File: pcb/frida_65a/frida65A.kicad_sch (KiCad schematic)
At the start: 44 parts, among them J1 CONN_PWR, J10 TP_LOGIC, J11 TP_OUT, J2 CONN_IN_P, J3 CONN_IN_N, J4 TP_CFG, J5 CONN_CFG, J6 TP_IN, J7 TP_INIT, J8 TP_SAMP, J9 TP_COMP, U1 DUT

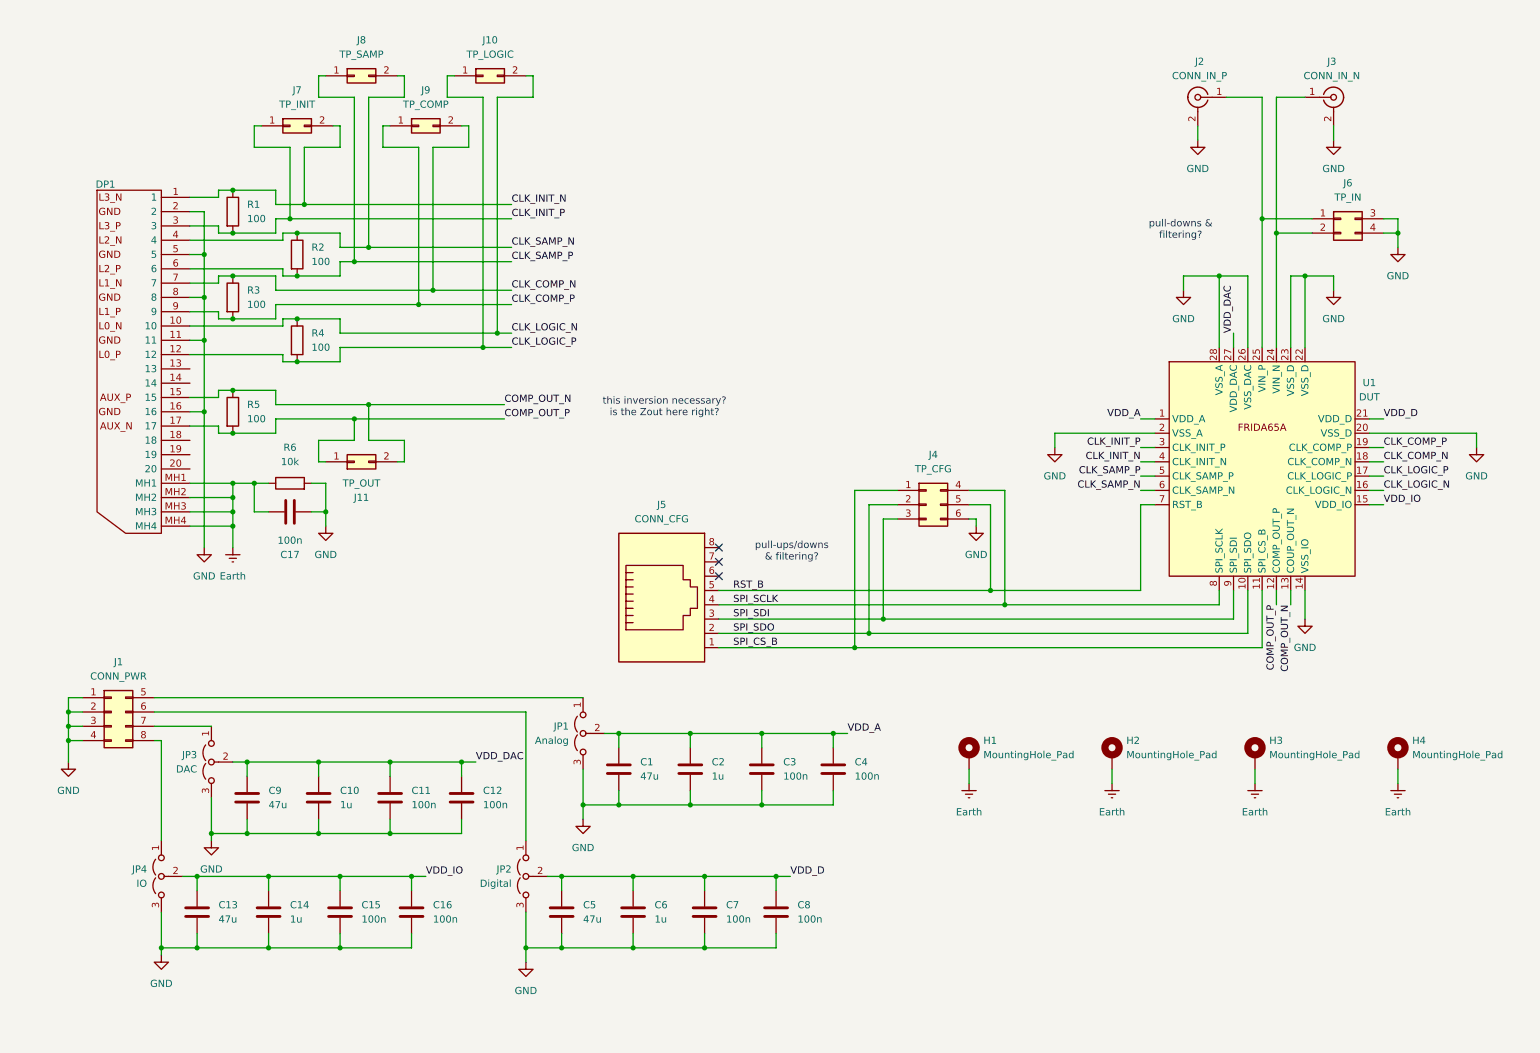
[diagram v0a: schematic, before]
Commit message: Update pcb
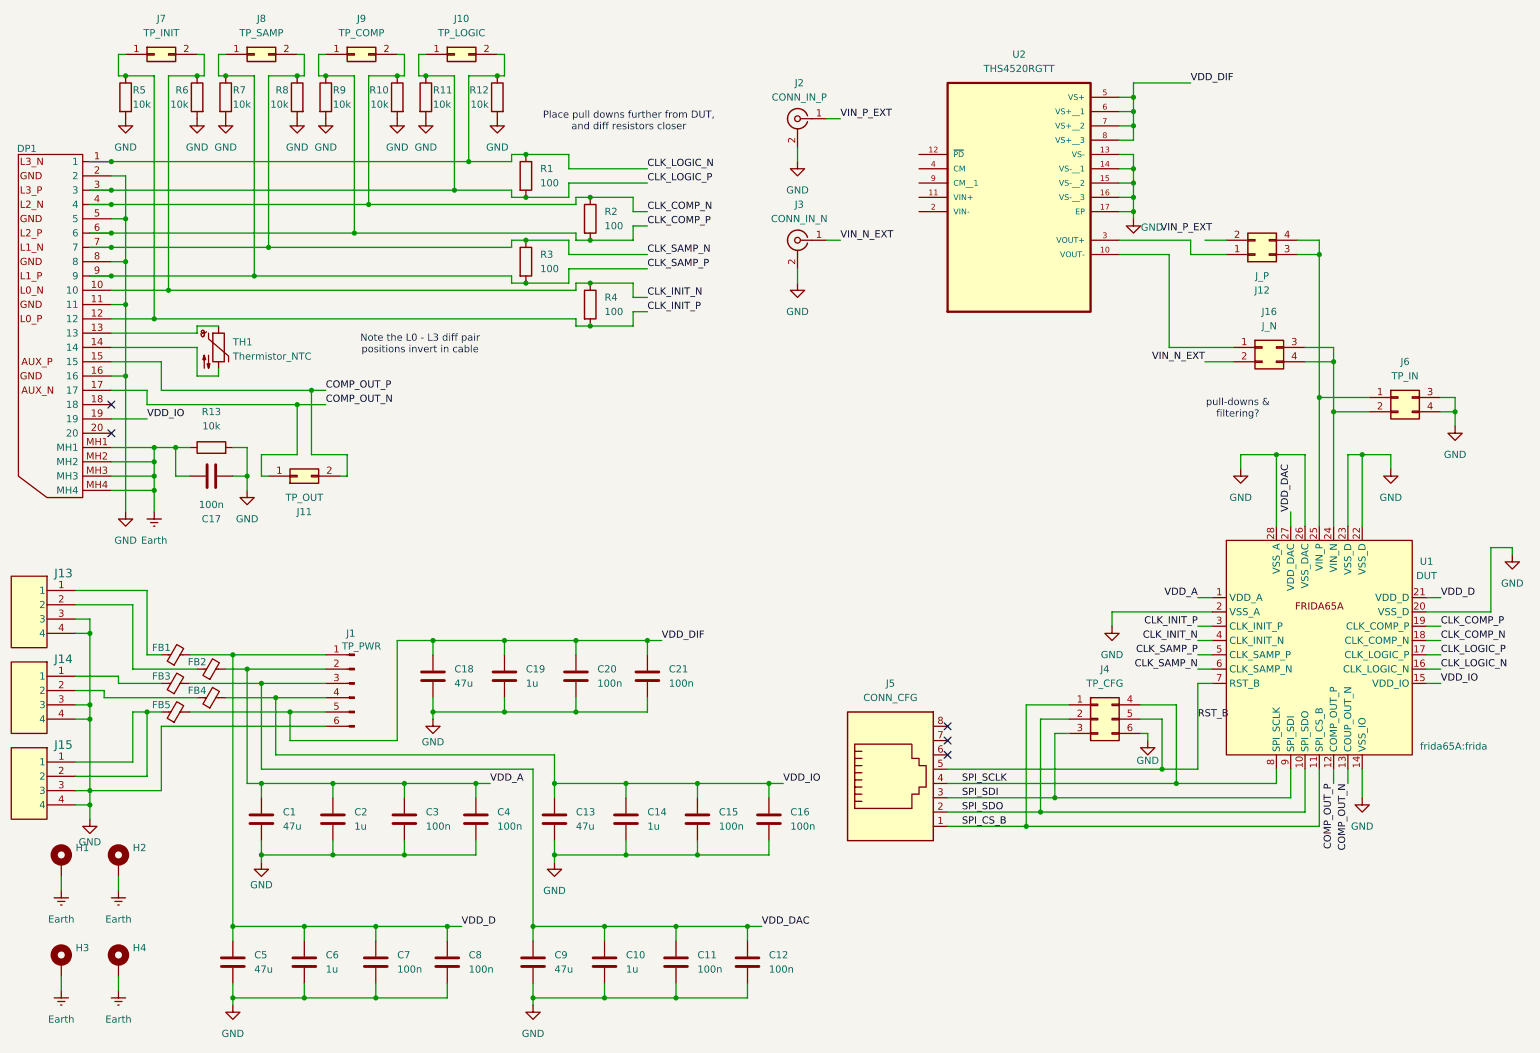
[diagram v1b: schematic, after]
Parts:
- removed J1: CONN_PWR, Silab:Molex_Mini-Fit_Jr_02x04_horizontal, symbol silab:Molex_02x04_Mini-Fit_Jr
- removed JP1: Analog, symbol Jumper:Jumper_3_Open
- removed JP2: Digital, symbol Jumper:Jumper_3_Open
- removed JP3: DAC, symbol Jumper:Jumper_3_Open
- removed JP4: IO, symbol Jumper:Jumper_3_Open
- added C18: 47u, Capacitor_SMD:C_0603_1608Metric, symbol Device:C
- added C19: 1u, Capacitor_SMD:C_0603_1608Metric, symbol Device:C
- added C20, C21: 100n, Capacitor_SMD:C_0603_1608Metric, symbol Device:C
- added FB1, FB2, FB3, FB4, FB5: FerriteBead_Small, Resistor_SMD:R_0603_1608Metric, symbol Device:FerriteBead_Small
- added J1: TP_PWR, Silab:Molex_Mini-Fit_Jr_02x04_horizontal, symbol Connector:Conn_01x06_Pin
- added J12: J_P, symbol Connector_Generic:Conn_02x02_Top_Bottom
- added J13, J14, J15: 469914004, CONN_SD-46991-001_04_MOL, symbol frida:469914004
- added J16: J_N, symbol Connector_Generic:Conn_02x02_Top_Bottom
- added R10, R11, R12, R6, R7, R8, R9: 10k, Resistor_SMD:R_0603_1608Metric, symbol Device:R
- added TH1: Thermistor_NTC, symbol Device:Thermistor_NTC
- added U2: THS4520RGTT, frida65A:QFN50P300X300X100-17N, symbol frida:THS4520RGTT
- C1, C10, C11, C12, C13, C14, C15, C16, C2, C3, C4, C5, C6, C7, C8, C9: footprint Capacitor_SMD:C_0201_0603Metric -> Capacitor_SMD:C_0603_1608Metric
- C17: footprint (none) -> Capacitor_SMD:C_0603_1608Metric
- DP1: footprint Silab:DP_Molex_47272-0024 -> silab:DP_Molex_47272-0024
- R1, R2, R3, R4: footprint (none) -> Resistor_SMD:R_0603_1608Metric
- R13: renamed from R6; footprint (none) -> Resistor_SMD:R_0603_1608Metric
- R5: value 100 -> 10k; footprint (none) -> Resistor_SMD:R_0603_1608Metric
- U1: footprint (none) -> frida65A:frida
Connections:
- net CLK_COMP_N: now also DP1.4, R2.1, R10.1; no longer DP1.7, R3.1
- net CLK_COMP_P: now also DP1.6, R2.2, R9.1; no longer DP1.9, R3.2
- net CLK_INIT_N: now also DP1.10, R4.1, R6.1; no longer DP1.1, R1.1
- net CLK_INIT_P: now also DP1.12, R4.2, R5.1; no longer DP1.3, R1.2
- net CLK_LOGIC_N: now also DP1.1, R1.1, R12.1; no longer DP1.10, R4.1
- net CLK_LOGIC_P: now also DP1.3, R1.2, R11.1; no longer DP1.12, R4.2
- net CLK_SAMP_N: now also DP1.7, R3.1, R8.1; no longer DP1.4, R2.1
- net CLK_SAMP_P: now also DP1.9, R3.2, R7.1; no longer DP1.6, R2.2
- net COMP_OUT_N: now also DP1.17, J11.1 (Pin_1); no longer DP1.15, J11.2 (Pin_2), R5.1
- net COMP_OUT_P: now also DP1.15, J11.2 (Pin_2); no longer DP1.17, J11.1 (Pin_1), R5.2
- net GND: now also R5.2, C18.2, C19.2, C20.2, C21.2, J1.6 (Pin_6), J13.3, J13.4, J14.3, J14.4, J15.3, J15.4, R10.2, R11.2, R12.2, R6.2, R7.2, R8.2, R9.2, U2.13 (VS-), U2.14 (VS-__1), U2.15 (VS-__2), U2.16 (VS-__3), U2.17 (EP)
- net VDD_A: now also FB2.2, J1.2 (Pin_2)
- net VDD_D: now also FB1.2, J1.1 (Pin_1)
- net VDD_DAC: now also FB3.2, J1.3 (Pin_3)
- net VDD_IO: now also DP1.19, FB4.2, J1.4 (Pin_4)
- net at J6.2 (Pin_2), U1.24 (VIN_N): now also J16.3 (Pin_3), J16.4 (Pin_4); no longer J3.1 (In)
- net at J6.1 (Pin_1), U1.25 (VIN_P): now also J12.3 (Pin_3), J12.4 (Pin_4); no longer J2.1 (In)
- net at DP1.13: now also TH1.1
- net at DP1.14: now also TH1.2
- new net: J16.1 (Pin_1), U2.10 (VOUT-)
- new net: J12.1 (Pin_1), U2.3 (VOUT+)
- new net: FB1.1, J13.1
- new net: FB2.1, J13.2
- new net: FB4.1, J14.2
- new net: FB5.1, J15.1, J15.2
- new net: FB3.1, J14.1
- new net VDD_DIF: C18.1, C19.1, C20.1, C21.1, FB5.2, J1.5 (Pin_5), U2.5 (VS+), U2.6 (VS+__1), U2.7 (VS+__2), U2.8 (VS+__3)
- new net VIN_N_EXT: J16.2 (Pin_2), J3.1 (In)
- new net VIN_P_EXT: J2.1 (In)
- no-connect marks 3 -> 5
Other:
- note added: "Note the L0 - L3 diff pair positions invert in cable"
- note added: "Place pull downs further from DUT, and diff resistors closer"
- note removed: "pull-ups/downs & filtering?"
- note removed: "this inversion necessary? is the Zout here right?"
- moved on the sheet: C1, C10, C11, C12, C13, C14, C15, C16, C17, C2, C3, C4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
